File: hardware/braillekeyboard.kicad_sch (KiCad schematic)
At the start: 10 parts, among them U1 74HCT237, U2 ESP32-C3-WROOM-02

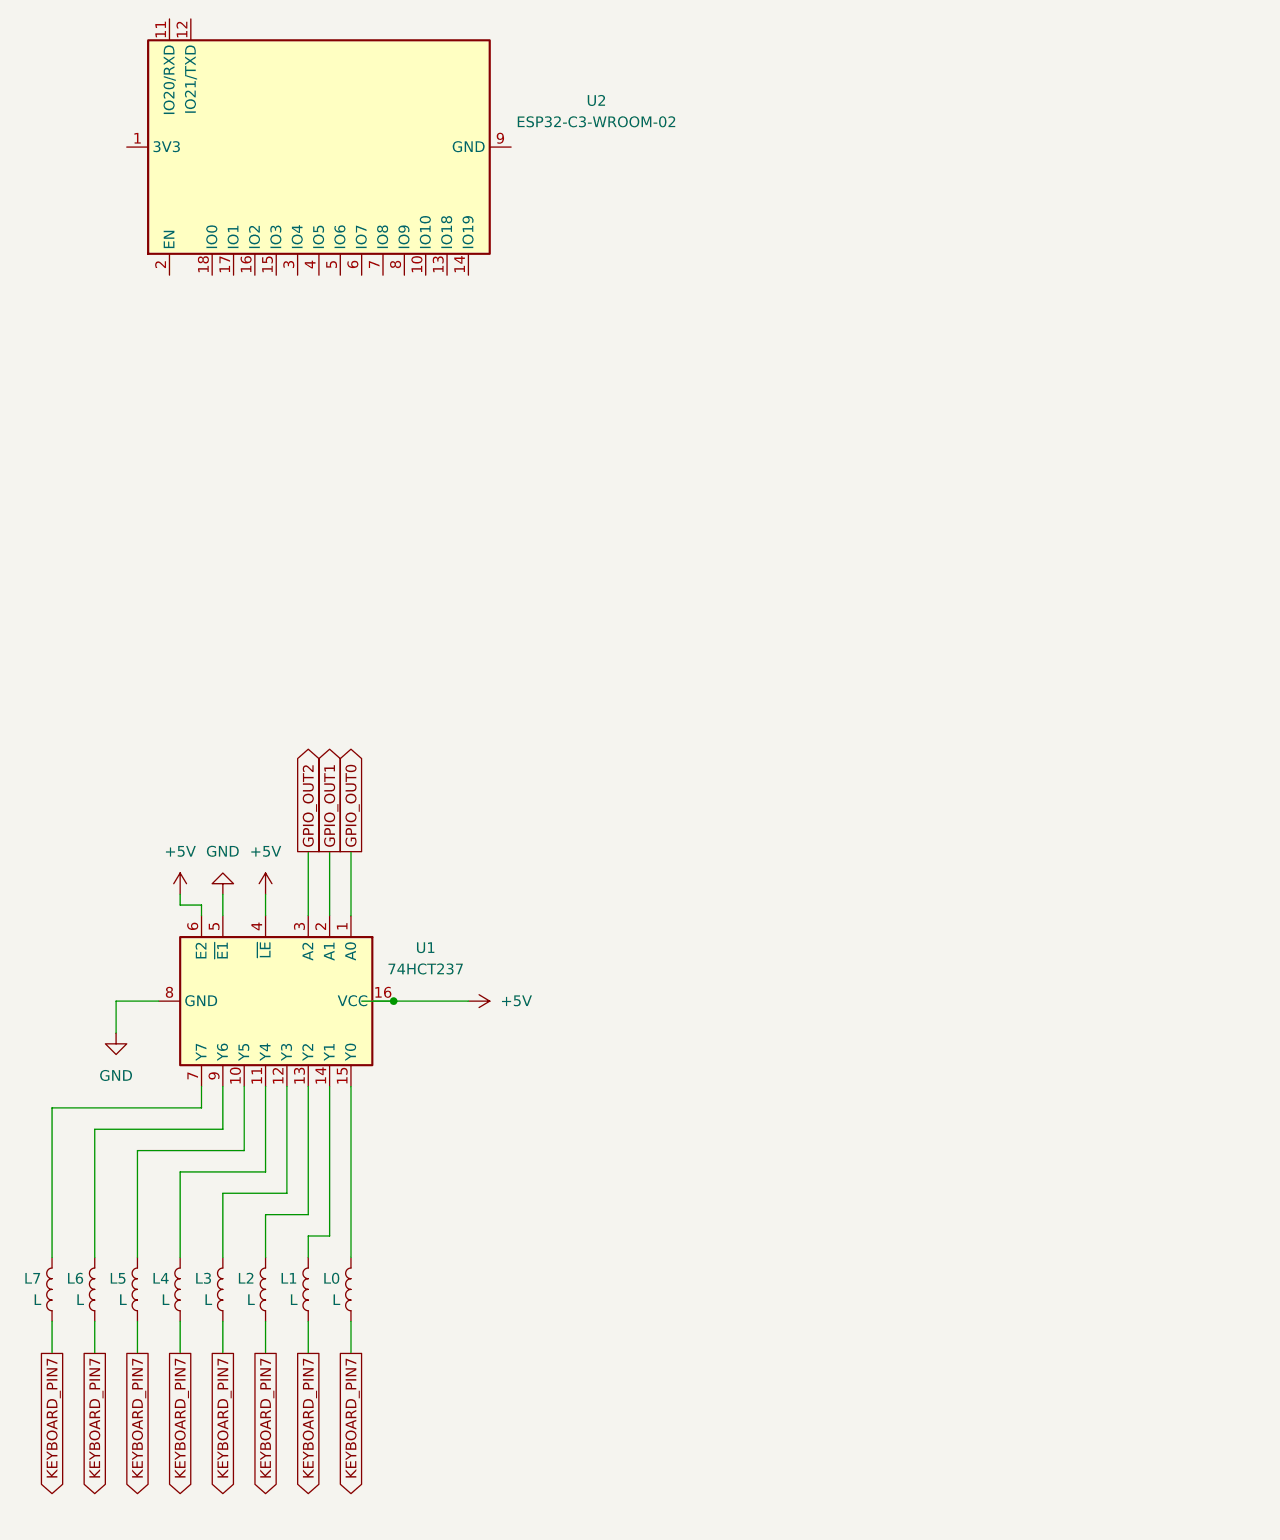
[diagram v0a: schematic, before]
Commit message: Schematic inclusion
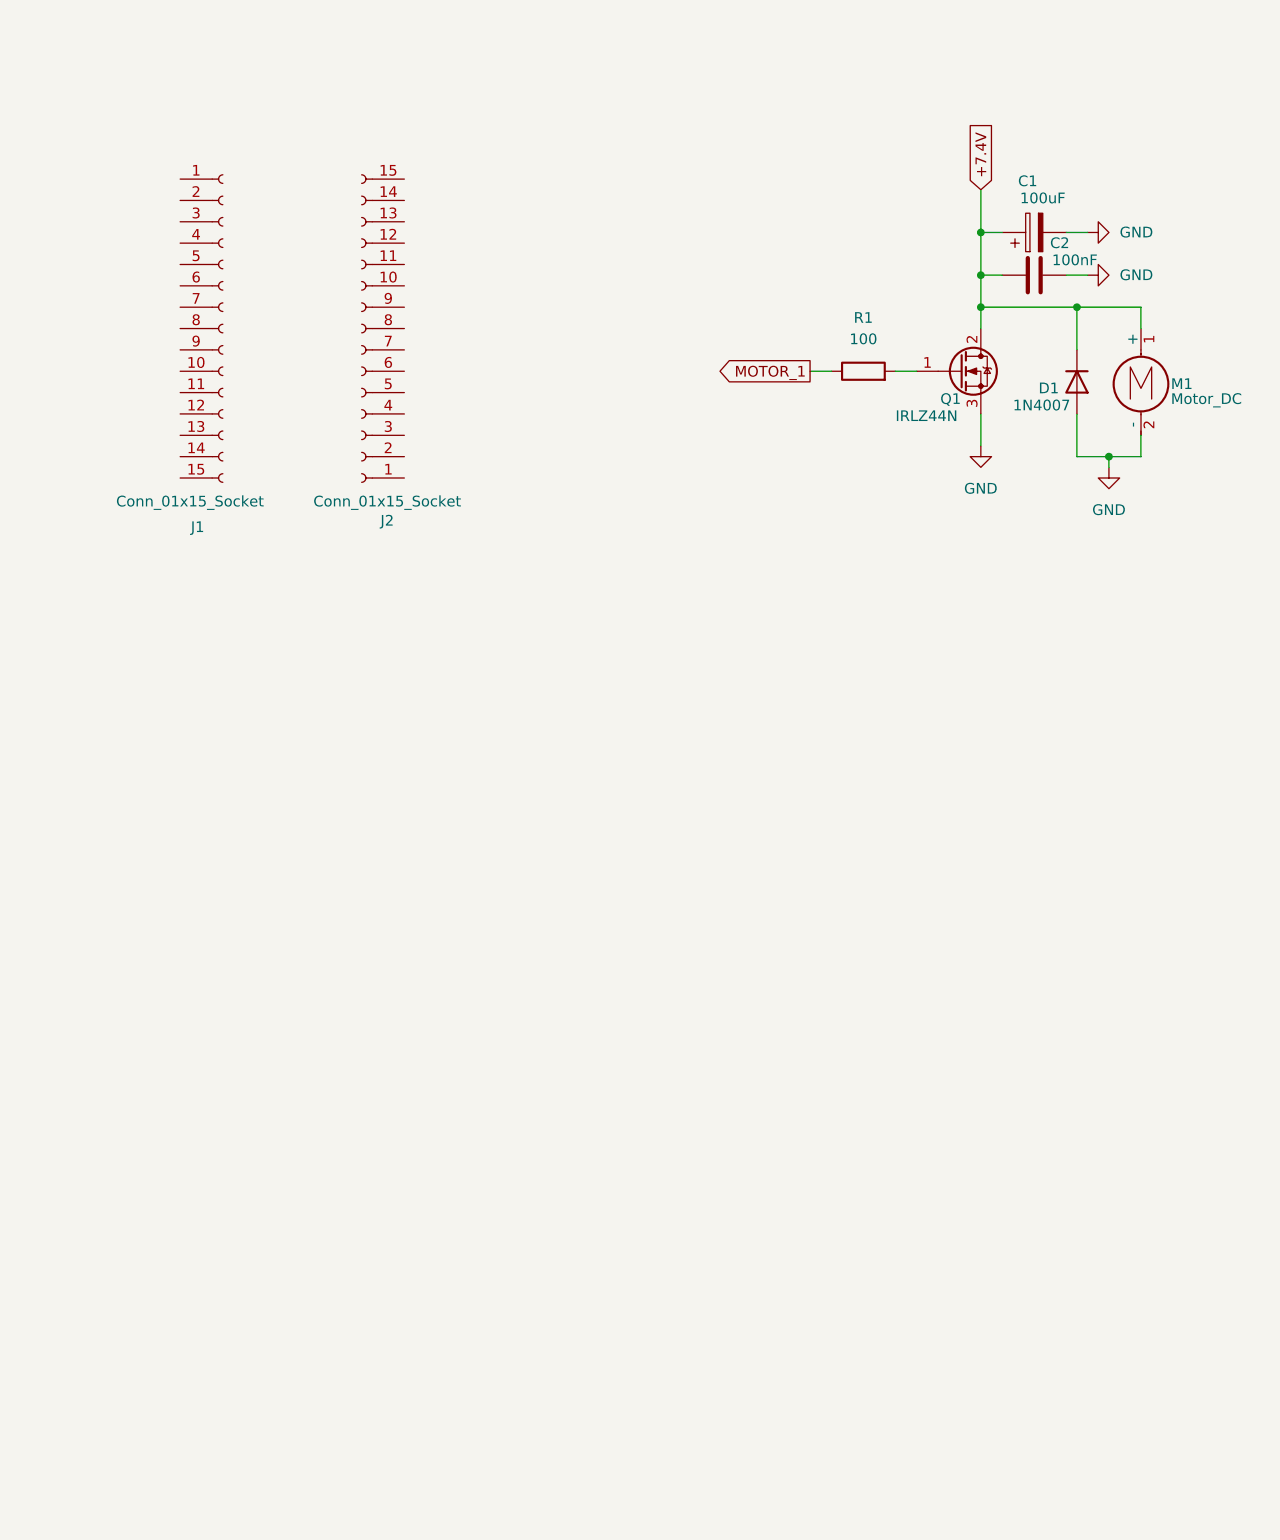
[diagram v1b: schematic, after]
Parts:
- removed L0, L1, L2, L3, L4, L5, L6, L7: L, symbol Device:L
- removed U1: 74HCT237, symbol 74xx:74HCT237
- removed U2: ESP32-C3-WROOM-02, RF_Module:ESP32-C3-WROOM-02, symbol RF_Module:ESP32-C3-WROOM-02
- added C1: 100uF, symbol Device:C_Polarized
- added C2: 100nF, symbol Device:C
- added D1: 1N4007, Diode_THT:D_DO-41_SOD81_P10.16mm_Horizontal, symbol Diode:1N4007
- added J1, J2: Conn_01x15_Socket, symbol Connector:Conn_01x15_Socket
- added M1: Motor_DC, symbol Motor:Motor_DC
- added Q1: IRLZ44N, Package_TO_SOT_THT:TO-220-3_Vertical, symbol Transistor_FET:IRLZ44N
- added R1: 100, symbol Device:R
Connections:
- net GND: now also C1.2, C2.2, D1.2 (A), M1.2 (-), Q1.3 (S)
- new net: Q1.1 (G), R1.2
- new net +7.4V: C1.1, C2.1, D1.1 (K), M1.1 (+), Q1.2 (D)
- new net MOTOR_1: R1.1
